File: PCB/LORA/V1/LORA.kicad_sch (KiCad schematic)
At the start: 15 parts, among them J1 Conn_02x06_Odd_Even, J2 Conn_02x06_Odd_Even, J3 Battery, Q1 NMOS, SW1 SW_SPDT, U1 RFM95CW

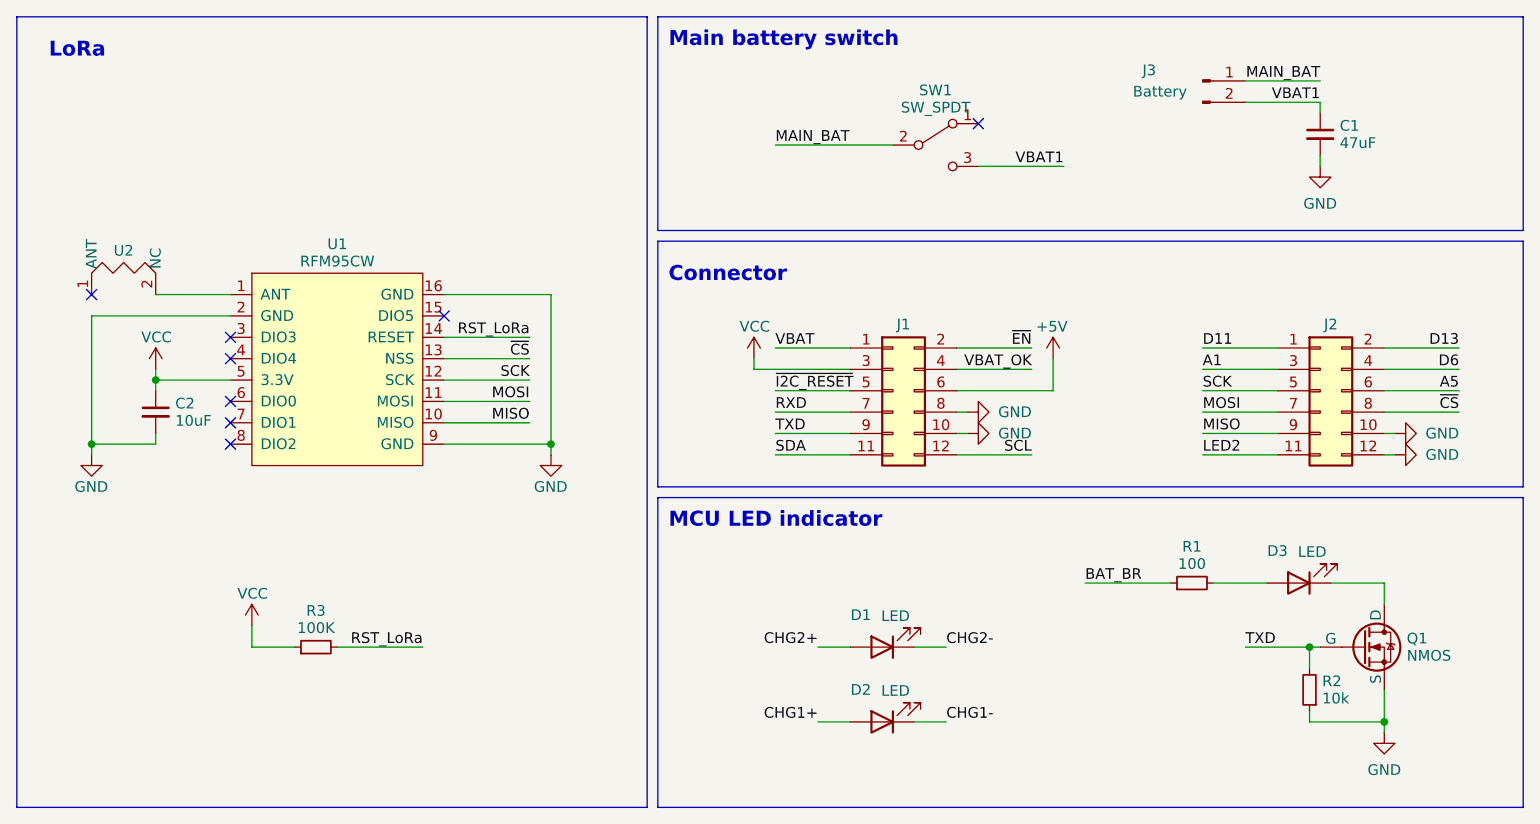
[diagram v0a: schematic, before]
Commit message: udated by FZ
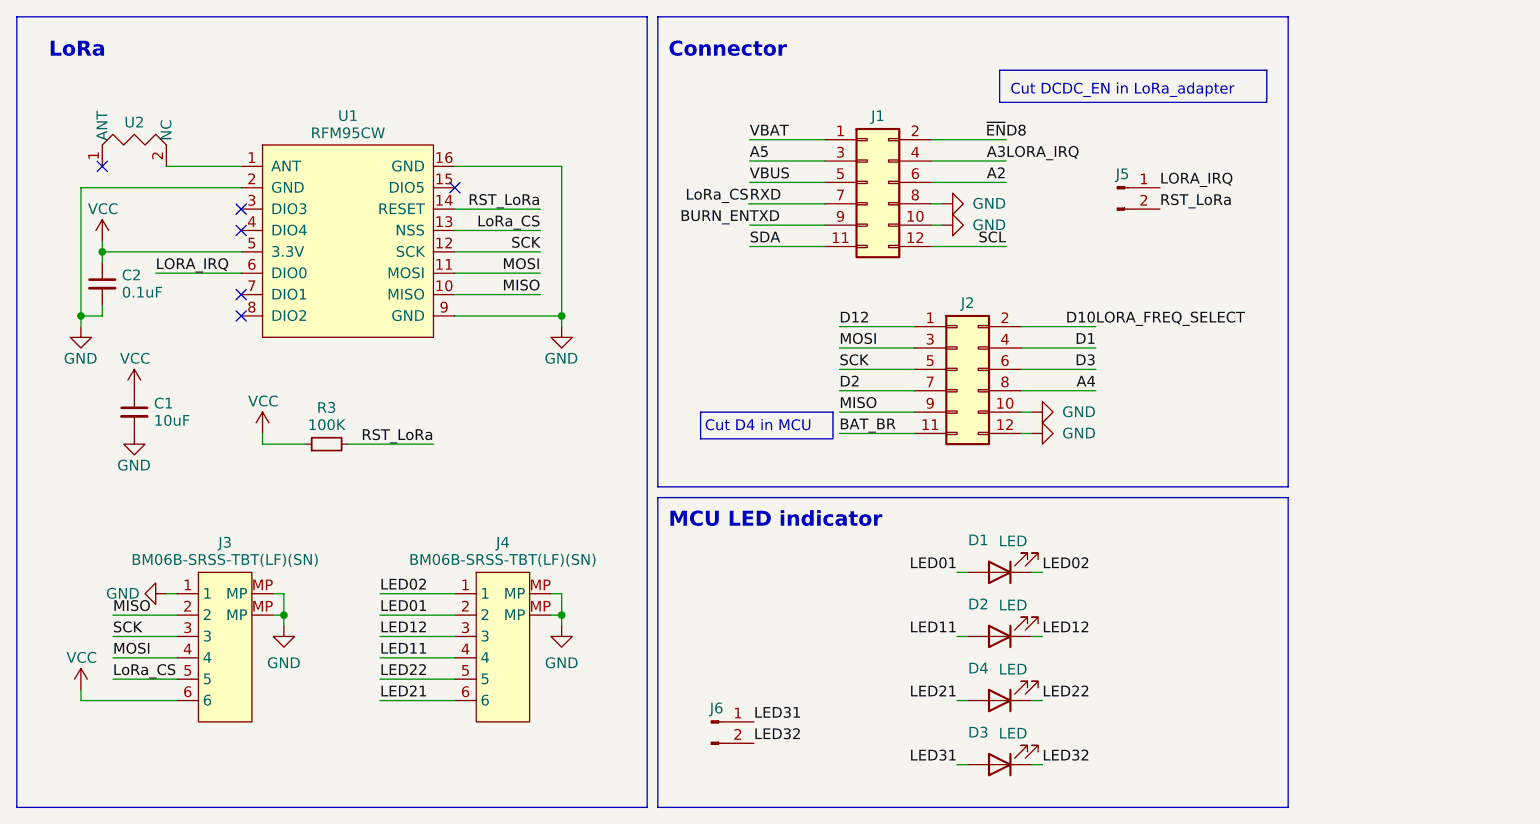
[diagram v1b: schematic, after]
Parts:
- removed J3: Battery, Connector_PinHeader_2.54mm:PinHeader_1x02_P2.54mm_Vertical, symbol Connector:Conn_01x02_Male
- removed Q1: NMOS, Package_TO_SOT_SMD:SOT-23, symbol Simulation_SPICE:NMOS
- removed R1: 100, Resistor_SMD:R_0603_1608Metric_Pad0.98x0.95mm_HandSolder, symbol Device:R_Small
- removed R2: 10k, Resistor_SMD:R_0603_1608Metric_Pad0.98x0.95mm_HandSolder, symbol Device:R_Small
- removed SW1: SW_SPDT, Connector_PinHeader_2.54mm:PinHeader_1x03_P2.54mm_Vertical, symbol Switch:SW_SPDT
- added D4: LED, LED_SMD:LED_0603_1608Metric_Pad1.05x0.95mm_HandSolder, symbol Device:LED
- added J3, J4: BM06B-SRSS-TBT(LF)(SN), Connector_JST:JST_SH_BM06B-SRSS-TB_1x06-1MP_P1.00mm_Vertical, symbol Mylib:BM06B-SURS-TF(LF)(SN)
- added J5, J6: Conn_01x02_Pin, Connector_PinHeader_2.00mm:PinHeader_1x02_P2.00mm_Vertical, symbol Connector:Conn_01x02_Pin
- C1: value 47uF -> 10uF; footprint Capacitor_Tantalum_SMD:CP_EIA-6032-15_Kemet-U_Pad2.25x2.35mm_HandSolder -> Capacitor_SMD:C_1206_3216Metric_Pad1.33x1.80mm_HandSolder
- C2: value 10uF -> 0.1uF
- D1, D2, D3: footprint LED_SMD:LED_1206_3216Metric_Pad1.42x1.75mm_HandSolder -> LED_SMD:LED_0603_1608Metric_Pad1.05x0.95mm_HandSolder
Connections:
- net A1 is gone; now on net MOSI: J2.3 (Pin_3)
- net LED2 is gone; now on net BAT_BR: J2.11 (Pin_11)
- net VBAT1 is gone; now on net VCC: C1.1
- net VBAT_OK is gone; now on net A3: J1.4 (Pin_4)
- net A5: now also J1.3 (Pin_3); no longer J2.6 (Pin_6)
- net GND: now also J3.1, J3.MP, J4.MP
- net MISO: now also J3.2
- net MOSI: now also J3.4; no longer J2.7 (Pin_7)
- net RST_LoRa: now also J5.2 (Pin_2)
- net SCK: now also J3.3
- net VCC: now also J3.6; no longer J1.3 (Pin_3)
- net LED32: now reaches D3.1 (K)
- net LED32: now also J6.2 (Pin_2)
- net LED31: now reaches D3.2 (A)
- net LED31: now also J6.1 (Pin_1)
- net A3: now reaches U1.6 (DIO0)
- net A3: now also J5.1 (Pin_1)
- net +5V renamed A2
- net CHG1+ renamed LED11
- net LED11: now also J4.4
- net CHG1- renamed LED12
- net LED12: now also J4.3
- net CHG2+ renamed LED01
- net LED01: now also J4.2
- net CHG2- renamed LED02
- net LED02: now also J4.1
- net D11 renamed D12
- net D13 renamed D10
- net D6 renamed D1
- net RXD renamed LoRa_CS
- net LoRa_CS: now also U1.13 (NSS), J3.5
- net TXD renamed BURN_EN
- net ~{CS} renamed A4
- net A4: no longer U1.13 (NSS)
- net ~{EN} renamed D8
- net ~{I2C_RESET} renamed VBUS
- new net D2: J2.7 (Pin_7)
- new net D3: J2.6 (Pin_6)
- new net LED21: D4.2 (A), J4.6
- new net LED22: D4.1 (K), J4.5
- no-connect marks 8 -> 6
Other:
- note added: "Cut D4 in MCU"
- note added: "Cut DCDC_EN in LoRa_adapter"
- note removed: "Main battery switch"
- moved on the sheet: C2, D1, J1, J2, R3, U1, U2
